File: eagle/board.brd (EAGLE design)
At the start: 57.5 x 49 mm, 31 parts

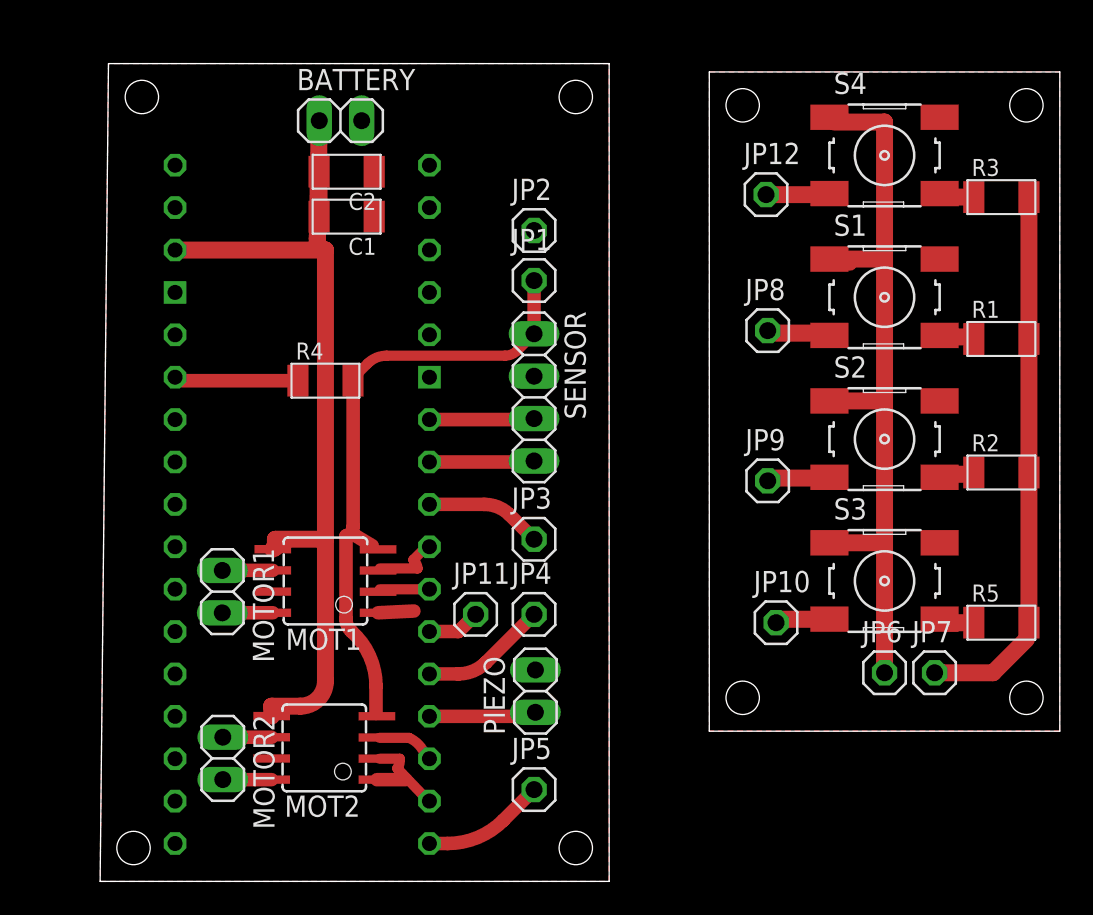
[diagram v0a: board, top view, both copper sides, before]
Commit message: added new picture
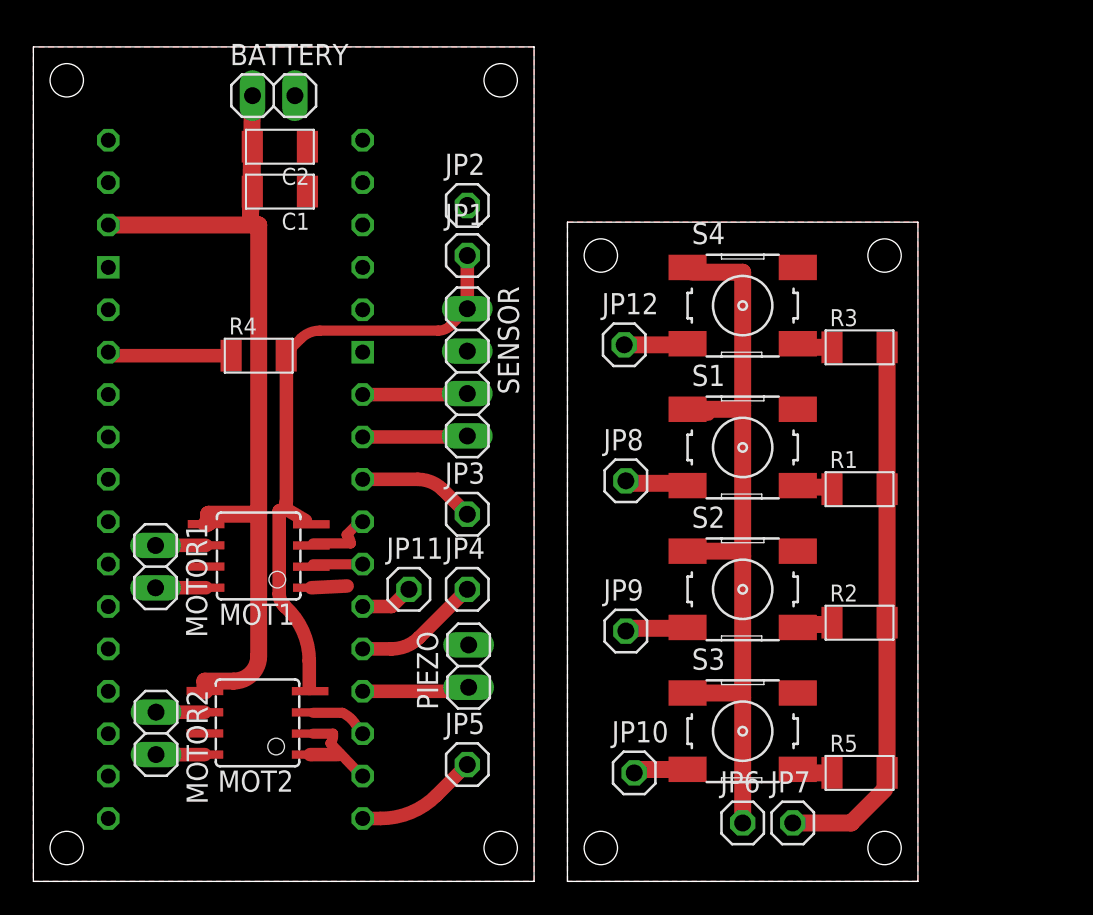
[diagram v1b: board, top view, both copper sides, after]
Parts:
- moved JP10 12.4 mm to (36.0, 6.50)
- moved JP12 12.4 mm to (35.4, 32.1)
- moved JP6 12.4 mm to (42.5, 3.50)
- moved JP7 12.4 mm to (45.5, 3.50)
- moved JP8 12.4 mm to (35.5, 24.0)
- moved JP9 12.4 mm to (35.5, 15.0)
- moved R1 12.4 mm to (49.5, 23.5)
- moved R2 12.4 mm to (49.5, 15.5)
- moved R3 12.4 mm to (49.5, 32.0)
- moved R5 12.4 mm to (49.5, 6.50)
- moved S1 12.4 mm to (42.5, 26.0)
- moved S2 12.4 mm to (42.5, 17.5)
- moved S3 12.4 mm to (42.5, 9.00)
- moved S4 12.4 mm to (42.5, 34.5)
- moved ARD 4.27 mm to (21.0, 2.50)
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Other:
- board size 57.5 x 49 mm -> 53 x 50 mm
